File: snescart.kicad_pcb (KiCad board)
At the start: 2 copper layers, 101.6 x 37.3 mm, 7 parts, among them P1 CASSETTE, U1 27C080

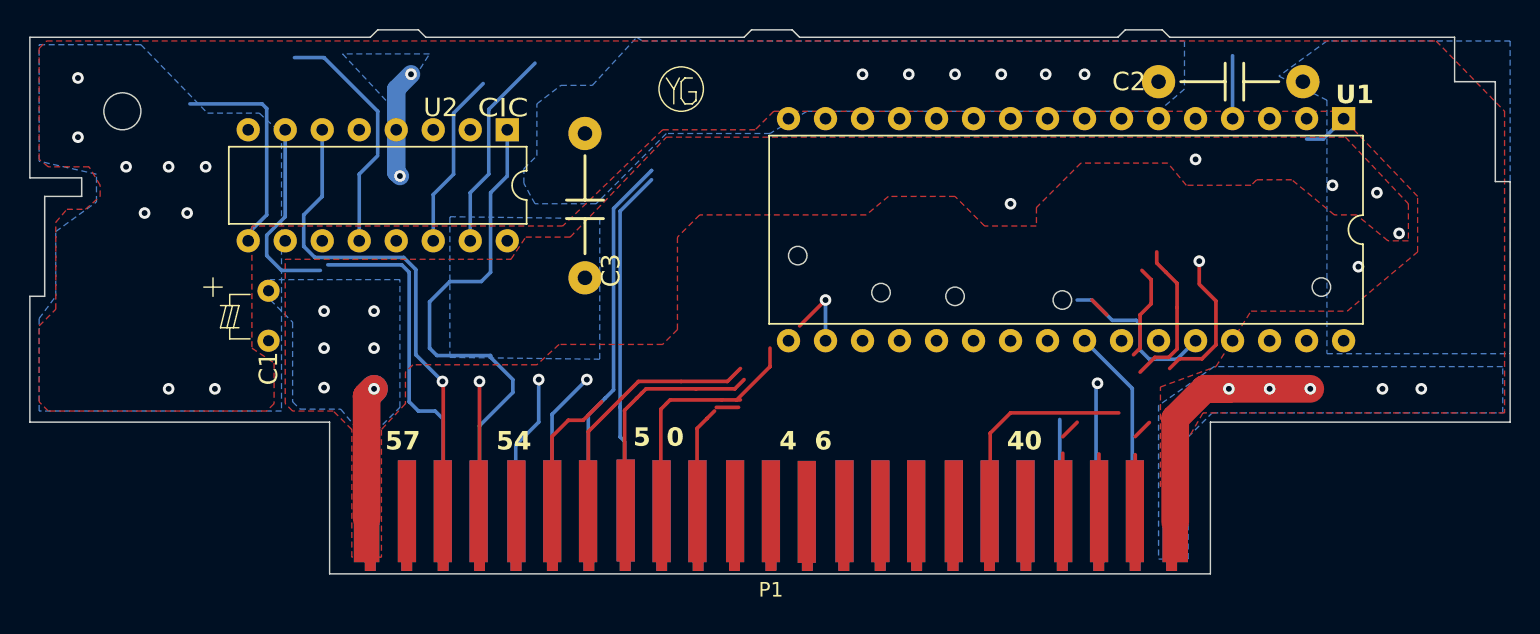
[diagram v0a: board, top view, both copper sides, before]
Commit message: track
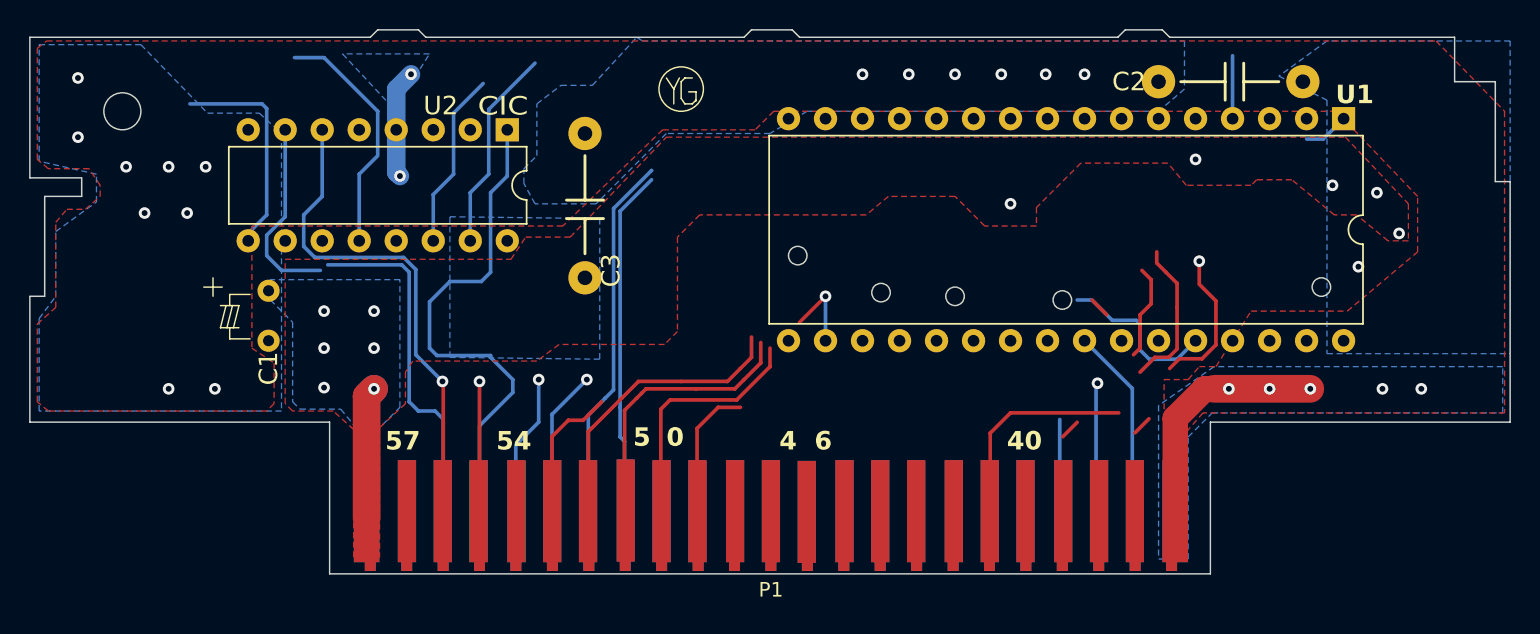
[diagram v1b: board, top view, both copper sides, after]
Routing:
- net Net-(P1-A14): track 12.7 -> 7.95 mm
- net Net-(P1-A13): track 26.5 -> 21.8 mm
- net Net-(P1-A12): track 20.6 -> 15.9 mm
- net Net-(P1-D5): track 16.7 -> 19.8 mm
- net Net-(P1-D6): track 18.4 -> 20.9 mm
- net GND: track 25.8 -> 25.0 mm
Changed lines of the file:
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@@
     (property "Sheetname" "")
     (attr through_hole)
-    (fp_text reference "U2" (at -1.524 4.572 180) (layer "F.SilkS")
+    (fp_text reference "U2" (at -1.651 4.572 180) (layer "F.SilkS")
         (effects (font (size 1.27 1.27) (thickness 0.15)))
     )
@@
     (effects (font (size 1.27 1.27) (thickness 0.3) bold) (justify left bottom))
   )
-  (gr_text "CIC" (at 124.714 118.618) (layer "F.SilkS")
+  (gr_text "CIC" (at 124.714 118.491) (layer "F.SilkS")
     (effects (font (size 1.27 1.5) (thickness 0.2)) (justify left bottom))
   )
@@
     (effects (font (size 1.27 1.27) (thickness 0.3) bold) (justify left bottom))
   )
-  (gr_text "SHVC-1AON-20" (at 98.552 115.57) (layer "F.Mask")
+  (gr_text "SHVC-1AON-20" (at 98.552 115.443) (layer "F.Mask")
     (effects (font (size 1.5 1.5) (thickness 0.3) bold) (justify left bottom))
   )
@@
     (effects (font (size 1.5 1.5) (thickness 0.3) bold) (justify left bottom))
   )
-  (segment (start 172.593 146.304) (end 172.593 139.192) (width 1.905) (layer "F.Cu") (net 1))
+  (segment (start 172.594 145.559) (end 172.594 139.191) (width 1.75) (layer "F.Cu") (net 1))
   (segment (start 175.26 137.16) (end 181.864 137.16) (width 1.905) (layer "F.Cu") (net 1))
-  (segment (start 172.593 139.192) (end 174.625 137.16) (width 1.905) (layer "F.Cu") (net 1))
-  (segment (start 174.625 137.16) (end 176.276 137.16) (width 1.905) (layer "F.Cu") (net 1))
+  (segment (start 172.594 139.191) (end 174.625 137.16) (width 1.75) (layer "F.Cu") (net 1))
+  (segment (start 174.625 137.16) (end 176.276 137.16) (width 1.75) (layer "F.Cu") (net 1))
   (via (at 97.282 115.824) (size 0.8) (drill 0.4) (layers "F.Cu" "B.Cu") (free) (net 1))
   (via (at 160.655 115.57) (size 0.8) (drill 0.4) (layers "F.Cu" "B.Cu") (free) (net 1))
@@
   (segment (start 125.476 122.428) (end 125.476 117.983) (width 0.25) (layer "B.Cu") (net 34))
   (segment (start 175.387 131.1275) (end 174.244 129.9845) (width 0.25) (layer "F.Cu") (net 35))
-  (segment (start 169.8498 140.4366) (end 170.815 139.4714) (width 0.254) (layer "F.Cu") (net 35))
+  (segment (start 169.8244 140.1826) (end 170.7896 139.2174) (width 0.254) (layer "F.Cu") (net 35))
   (segment (start 174.432991 135.097004) (end 172.877996 135.097004) (width 0.25) (layer "F.Cu") (net 35))
   (segment (start 174.244 128.143) (end 174.244 129.921) (width 0.25) (layer "F.Cu") (net 35))
   (segment (start 175.387 134.142995) (end 175.387 131.1275) (width 0.25) (layer "F.Cu") (net 35))
   (segment (start 172.877996 135.097004) (end 172.212 135.763) (width 0.25) (layer "F.Cu") (net 35))
-  (segment (start 169.8498 146.304) (end 169.8498 141.6812) (width 0.254) (layer "F.Cu") (net 35))
   (segment (start 174.432991 135.097004) (end 175.387 134.142995) (width 0.25) (layer "F.Cu") (net 35))
   (via (at 174.244 128.397) (size 0.8) (drill 0.4) (layers "F.Cu" "B.Cu") (net 35))
@@
   (segment (start 171.196 135.001) (end 170.18 136.017) (width 0.25) (layer "F.Cu") (net 36))
   (segment (start 171.323 128.524) (end 171.323 127.762) (width 0.25) (layer "F.Cu") (net 36))
-  (segment (start 167.3606 146.304) (end 167.3606 141.6304) (width 0.254) (layer "F.Cu") (net 36))
   (segment (start 172.72 134.427991) (end 172.146991 135.001) (width 0.25) (layer "F.Cu") (net 36))
   (segment (start 172.72 129.921) (end 171.958 129.159) (width 0.25) (layer "F.Cu") (net 36))
@@
   (segment (start 170.18 134.493) (end 170.18 132.715) (width 0.25) (layer "B.Cu") (net 36))
   (segment (start 170.18 132.969) (end 170.18 132.08) (width 0.254) (layer "F.Cu") (net 37))
-  (segment (start 164.8714 146.304) (end 164.8714 141.5796) (width 0.254) (layer "F.Cu") (net 37))
   (segment (start 170.942 131.318) (end 170.942 129.667) (width 0.254) (layer "F.Cu") (net 37))
   (segment (start 170.18 134.366) (end 170.18 132.969) (width 0.254) (layer "F.Cu") (net 37))
@@
   (segment (start 184.15 118.618) (end 182.753 120.015) (width 0.254) (layer "B.Cu") (net 42))
   (segment (start 182.753 120.015) (end 181.61 120.015) (width 0.254) (layer "B.Cu") (net 42))
-  (segment (start 140.462 139.192) (end 140.97 138.684) (width 0.254) (layer "F.Cu") (net 43))
-  (segment (start 139.7762 139.8778) (end 140.462 139.192) (width 0.254) (layer "F.Cu") (net 43))
-  (segment (start 141.097 138.43) (end 142.621 138.43) (width 0.254) (layer "F.Cu") (net 43))
+  (segment (start 139.7762 139.8778) (end 141.224 138.43) (width 0.254) (layer "F.Cu") (net 43))
   (segment (start 139.7762 146.304) (end 139.7762 139.8778) (width 0.254) (layer "F.Cu") (net 43))
-  (segment (start 137.287 138.557) (end 137.668 138.176) (width 0.25) (layer "F.Cu") (net 44))
-  (segment (start 141.478 137.922) (end 142.748 137.922) (width 0.25) (layer "F.Cu") (net 44))
-  (segment (start 137.922 137.922) (end 141.478 137.922) (width 0.25) (layer "F.Cu") (net 44))
-  (segment (start 137.668 138.176) (end 137.922 137.922) (width 0.25) (layer "F.Cu") (net 44))
-  (segment (start 142.494 137.922) (end 144.78 135.636) (width 0.25) (layer "F.Cu") (net 44))
-  (segment (start 146.812 132.842) (end 148.59 131.064) (width 0.25) (layer "F.Cu") (net 44))
-  (segment (start 144.78 135.636) (end 144.78 134.366) (width 0.25) (layer "F.Cu") (net 44))
-  (segment (start 137.287 146.304) (end 137.287 138.557) (width 0.25) (layer "F.Cu") (net 44))
-  (via (at 148.59 131.064) (size 0.8) (drill 0.4) (layers "F.Cu" "B.Cu") (net 44))
-  (segment (start 148.59 131.064) (end 148.59 133.858) (width 0.254) (layer "B.Cu") (net 44))
+  (segment (start 141.224 138.43) (end 142.748 138.43) (width 0.254) (layer "F.Cu") (net 43))
+  (segment (start 137.287 138.557) (end 137.287 146.304) (width 0.25) (layer "F.Cu") (net 44))
+  (segment (start 142.494 137.922) (end 137.922 137.922) (width 0.25) (layer "F.Cu") (net 44))
+  (segment (start 144.78 134.366) (end 144.78 135.636) (width 0.25) (layer "F.Cu") (net 44))
+  (segment (start 146.812 132.588) (end 148.59 130.81) (width 0.25) (layer "F.Cu") (net 44))
+  (segment (start 144.78 135.636) (end 142.494 137.922) (width 0.25) (layer "F.Cu") (net 44))
+  (segment (start 137.922 137.922) (end 137.287 138.557) (width 0.25) (layer "F.Cu") (net 44))
+  (via (at 148.59 130.81) (size 0.8) (drill 0.4) (layers "F.Cu" "B.Cu") (net 44))
+  (segment (start 148.59 130.81) (end 148.59 133.604) (width 0.254) (layer "B.Cu") (net 44))
   (segment (start 135.961 137.47) (end 136.271 137.16) (width 0.254) (layer "F.Cu") (net 45))
   (segment (start 139.7 137.16) (end 142.367 137.16) (width 0.254) (layer "F.Cu") (net 45))
   (segment (start 134.7978 146.304) (end 134.7978 138.6332) (width 0.254) (layer "F.Cu") (net 45))
+  (segment (start 144.145 135.382) (end 144.145 133.985) (width 0.254) (layer "F.Cu") (net 45))
   (segment (start 136.271 137.16) (end 139.7 137.16) (width 0.254) (layer "F.Cu") (net 45))
+  (segment (start 143.002 136.525) (end 144.145 135.382) (width 0.254) (layer "F.Cu") (net 45))
   (segment (start 135.636 137.795) (end 135.961 137.47) (width 0.254) (layer "F.Cu") (net 45))
   (segment (start 134.7978 138.6332) (end 135.636 137.795) (width 0.254) (layer "F.Cu") (net 45))
   (segment (start 142.367 137.16) (end 143.002 136.525) (width 0.254) (layer "F.Cu") (net 45))
+  (segment (start 143.51 135.001) (end 143.51 133.604) (width 0.254) (layer "F.Cu") (net 48))
   (segment (start 132.3086 140.0937) (end 132.3086 146.304) (width 0.254) (layer "F.Cu") (net 48))
   (segment (start 135.7503 136.652) (end 138.684 136.652) (width 0.254) (layer "F.Cu") (net 48))
   (segment (start 132.3086 140.0937) (end 134.62 137.7823) (width 0.254) (layer "F.Cu") (net 48))
+  (segment (start 142.748 135.763) (end 143.51 135.001) (width 0.254) (layer "F.Cu") (net 48))
   (segment (start 141.859 136.652) (end 142.748 135.763) (width 0.254) (layer "F.Cu") (net 48))
   (segment (start 138.684 136.652) (end 141.859 136.652) (width 0.254) (layer "F.Cu") (net 48))
@@
     (polygon
       (pts
-        (xy 116.078 148.717)
-        (xy 116.078 139.954)
+        (xy 116.205 148.717)
+        (xy 116.205 139.954)
         (xy 114.808 138.684)
         (xy 112.014 138.684)
@@
         (xy 139.954 125.222)
         (xy 138.43 126.746)
-        (xy 138.43 133.096)
-        (xy 137.414 134.112)
+        (xy 138.43 133.223)
+        (xy 137.541 134.112)
         (xy 130.302 134.112)
-        (xy 128.778 135.509)
-        (xy 120.269 135.509)
+        (xy 128.778 135.255)
+        (xy 120.269 135.255)
         (xy 119.761 136.017)
         (xy 119.761 138.176)
-        (xy 118.11 139.954)
-        (xy 118.11 148.717)
+        (xy 117.983 139.827)
+        (xy 117.983 148.717)
       )
     )
@@
     (polygon
       (pts
-        (xy 94.615 138.049)
-        (xy 94.615 132.842)
-        (xy 95.758 131.699)
+        (xy 94.488 138.049)
+        (xy 94.488 132.715)
+        (xy 95.758 131.572)
         (xy 95.758 125.73)
         (xy 96.52 124.841)
@@
         (xy 98.806 123.952)
         (xy 98.806 123.19)
-        (xy 98.044 121.92)
-        (xy 95.25 121.92)
-        (xy 94.615 121.412)
-        (xy 94.615 113.792)
+        (xy 98.044 122.047)
+        (xy 95.25 122.047)
+        (xy 94.488 121.412)
+        (xy 94.488 113.792)
         (xy 95.123 113.284)
         (xy 190.5 113.284)
@@
         (xy 195.199 138.811)
         (xy 174.498 138.811)
-        (xy 171.577 143.891)
-        (xy 171.577 137.033)
+        (xy 171.831 141.859)
+        (xy 171.831 136.525)
+        (xy 173.482 136.525)
+        (xy 174.244 135.636)
         (xy 175.387 135.636)
         (xy 177.8 131.826)

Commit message: track club
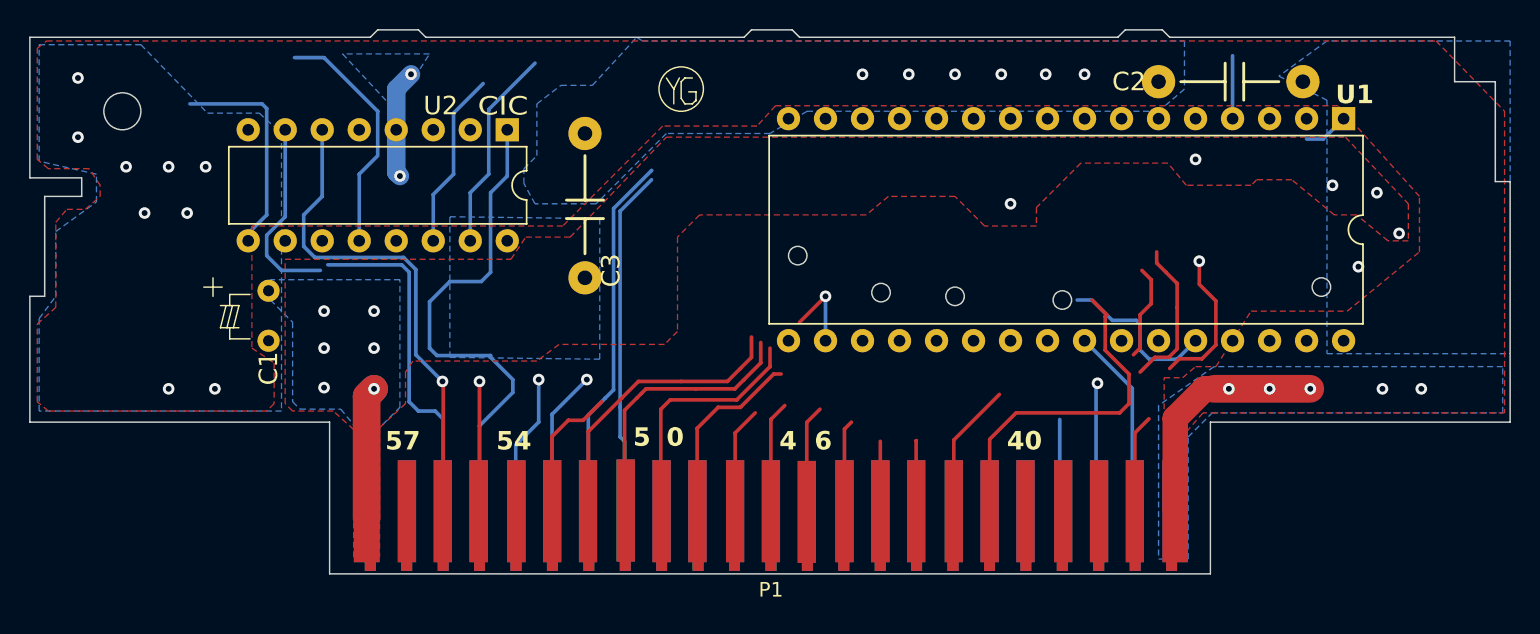
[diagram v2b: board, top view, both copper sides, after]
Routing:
- net Net-(P1-A17): track 0.00 -> 9.31 mm
- net unconnected-(P1-A22-Pad47): track 0.00 -> 7.65 mm
- net unconnected-(P1-A21-Pad46): track 0.00 -> 7.42 mm
- net unconnected-(P1-A23-Pad48): track 0.00 -> 7.32 mm
- net Net-(P1-A16): track 16.9 -> 23.8 mm
- net unconnected-(P1-A20-Pad45): track 0.00 -> 6.31 mm
- net Net-(P1-A12): track 15.9 -> 21.3 mm
- net Net-(P1-A18): track 0.00 -> 4.84 mm
- net Net-(P1-A19): track 3.12 -> 7.91 mm
- net unconnected-(P1-ROMSEL-Pad49): track 10.00 -> 13.7 mm
- net Net-(P1-A14): track 7.95 -> 6.55 mm
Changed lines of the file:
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@@
   (segment (start 174.432991 135.097004) (end 172.877996 135.097004) (width 0.25) (layer "F.Cu") (net 35))
   (segment (start 174.244 128.143) (end 174.244 129.921) (width 0.25) (layer "F.Cu") (net 35))
+  (segment (start 169.825 140.1832) (end 169.8244 140.1826) (width 0.25) (layer "F.Cu") (net 35))
   (segment (start 175.387 134.142995) (end 175.387 131.1275) (width 0.25) (layer "F.Cu") (net 35))
   (segment (start 172.877996 135.097004) (end 172.212 135.763) (width 0.25) (layer "F.Cu") (net 35))
   (segment (start 174.432991 135.097004) (end 175.387 134.142995) (width 0.25) (layer "F.Cu") (net 35))
+  (segment (start 169.825 145.559) (end 169.825 140.1832) (width 0.25) (layer "F.Cu") (net 35))
   (via (at 174.244 128.397) (size 0.8) (drill 0.4) (layers "F.Cu" "B.Cu") (net 35))
   (segment (start 176.53 118.618) (end 176.53 114.3) (width 0.254) (layer "B.Cu") (net 35))
@@
   (segment (start 170.18 132.08) (end 170.942 131.318) (width 0.254) (layer "F.Cu") (net 37))
   (segment (start 170.942 129.667) (end 170.307 129.032) (width 0.254) (layer "F.Cu") (net 37))
-  (segment (start 164.8714 140.4493) (end 165.862 139.4587) (width 0.254) (layer "F.Cu") (net 37))
+  (segment (start 161.671 138.811) (end 168.783 138.811) (width 0.25) (layer "F.Cu") (net 39))
+  (segment (start 167.785 132.189) (end 167.894 132.08) (width 0.25) (layer "F.Cu") (net 39))
+  (segment (start 167.785 134.511) (end 167.785 132.189) (width 0.25) (layer "F.Cu") (net 39))
+  (segment (start 168.783 138.811) (end 169.418 138.176) (width 0.25) (layer "F.Cu") (net 39))
+  (segment (start 169.418 138.176) (end 169.418 136.144) (width 0.25) (layer "F.Cu") (net 39))
+  (segment (start 159.858 140.624) (end 161.671 138.811) (width 0.25) (layer "F.Cu") (net 39))
+  (segment (start 159.858 145.559) (end 159.858 140.624) (width 0.25) (layer "F.Cu") (net 39))
   (segment (start 167.894 132.08) (end 166.878 131.064) (width 0.25) (layer "F.Cu") (net 39))
-  (segment (start 161.29 138.811) (end 159.893 140.208) (width 0.25) (layer "F.Cu") (net 39))
-  (segment (start 161.29 138.811) (end 168.714 138.811) (width 0.25) (layer "F.Cu") (net 39))
-  (segment (start 159.893 140.208) (end 159.893 146.304) (width 0.25) (layer "F.Cu") (net 39))
+  (segment (start 169.418 136.144) (end 167.785 134.511) (width 0.25) (layer "F.Cu") (net 39))
+  (segment (start 157.398 145.559) (end 157.398 140.671) (width 0.25) (layer "F.Cu") (net 40))
+  (segment (start 157.398 140.671) (end 160.528 137.541) (width 0.25) (layer "F.Cu") (net 40))
+  (segment (start 154.811 140.718) (end 154.813 140.716) (width 0.25) (layer "F.Cu") (net 41))
+  (segment (start 154.811 145.559) (end 154.811 140.718) (width 0.25) (layer "F.Cu") (net 41))
+  (segment (start 152.351 145.559) (end 152.351 140.765) (width 0.25) (layer "F.Cu") (net 42))
   (via (at 185.166 128.778) (size 0.8) (drill 0.4) (layers "F.Cu" "B.Cu") (net 42))
   (segment (start 184.15 118.618) (end 182.753 120.015) (width 0.254) (layer "B.Cu") (net 42))
   (segment (start 182.753 120.015) (end 181.61 120.015) (width 0.254) (layer "B.Cu") (net 42))
   (segment (start 139.7762 139.8778) (end 141.224 138.43) (width 0.254) (layer "F.Cu") (net 43))
+  (segment (start 145.034 136.144) (end 145.542 136.144) (width 0.254) (layer "F.Cu") (net 43))
   (segment (start 139.7762 146.304) (end 139.7762 139.8778) (width 0.254) (layer "F.Cu") (net 43))
   (segment (start 141.224 138.43) (end 142.748 138.43) (width 0.254) (layer "F.Cu") (net 43))
+  (segment (start 142.748 138.43) (end 145.034 136.144) (width 0.254) (layer "F.Cu") (net 43))
   (segment (start 137.287 138.557) (end 137.287 146.304) (width 0.25) (layer "F.Cu") (net 44))
   (segment (start 142.494 137.922) (end 137.922 137.922) (width 0.25) (layer "F.Cu") (net 44))
@@
   (segment (start 129.8194 140.4366) (end 129.8194 146.304) (width 0.254) (layer "F.Cu") (net 49))
   (segment (start 131.953 139.319) (end 133.223 138.049) (width 0.254) (layer "F.Cu") (net 49))
+  (segment (start 149.891 145.559) (end 149.891 139.923) (width 0.25) (layer "F.Cu") (net 52))
+  (segment (start 149.891 139.923) (end 150.368 139.446) (width 0.25) (layer "F.Cu") (net 52))
+  (segment (start 147.304 145.607) (end 147.304 139.462) (width 0.25) (layer "F.Cu") (net 53))
+  (segment (start 147.304 139.462) (end 148.209 138.557) (width 0.25) (layer "F.Cu") (net 53))
+  (segment (start 144.844 139.255) (end 145.796 138.303) (width 0.25) (layer "F.Cu") (net 54))
+  (segment (start 144.844 145.559) (end 144.844 139.255) (width 0.25) (layer "F.Cu") (net 54))
+  (segment (start 142.384 140.191) (end 143.764 138.811) (width 0.25) (layer "F.Cu") (net 55))
+  (segment (start 142.384 145.559) (end 142.384 140.191) (width 0.25) (layer "F.Cu") (net 55))
   (zone (net 2) (net_name "VCC") (layer "F.Cu") (hatch edge 0.5)
     (priority 2)
@@
         (xy 174.498 138.811)
         (xy 171.831 141.859)
-        (xy 171.831 136.525)
-        (xy 173.482 136.525)
-        (xy 174.244 135.636)
+        (xy 171.831 136.398)
+        (xy 173.101 136.398)
+        (xy 173.99 135.636)
         (xy 175.387 135.636)
         (xy 177.8 131.826)
         (xy 184.404 131.826)
-        (xy 189.23 127.762)
-        (xy 189.23 123.952)
-        (xy 183.642 118.11)
-        (xy 145.034 118.11)
-        (xy 143.764 119.38)
-        (xy 137.414 119.38)
+        (xy 189.357 127.762)
+        (xy 189.357 123.952)
+        (xy 183.769 117.729)
+        (xy 145.161 117.729)
+        (xy 143.891 119.126)
+        (xy 137.414 119.126)
         (xy 130.556 125.984)
         (xy 109.22 125.984)
